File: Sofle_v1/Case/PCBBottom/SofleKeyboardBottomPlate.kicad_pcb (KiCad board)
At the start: 2 copper layers, 137.2 x 109.2 mm, 9 parts

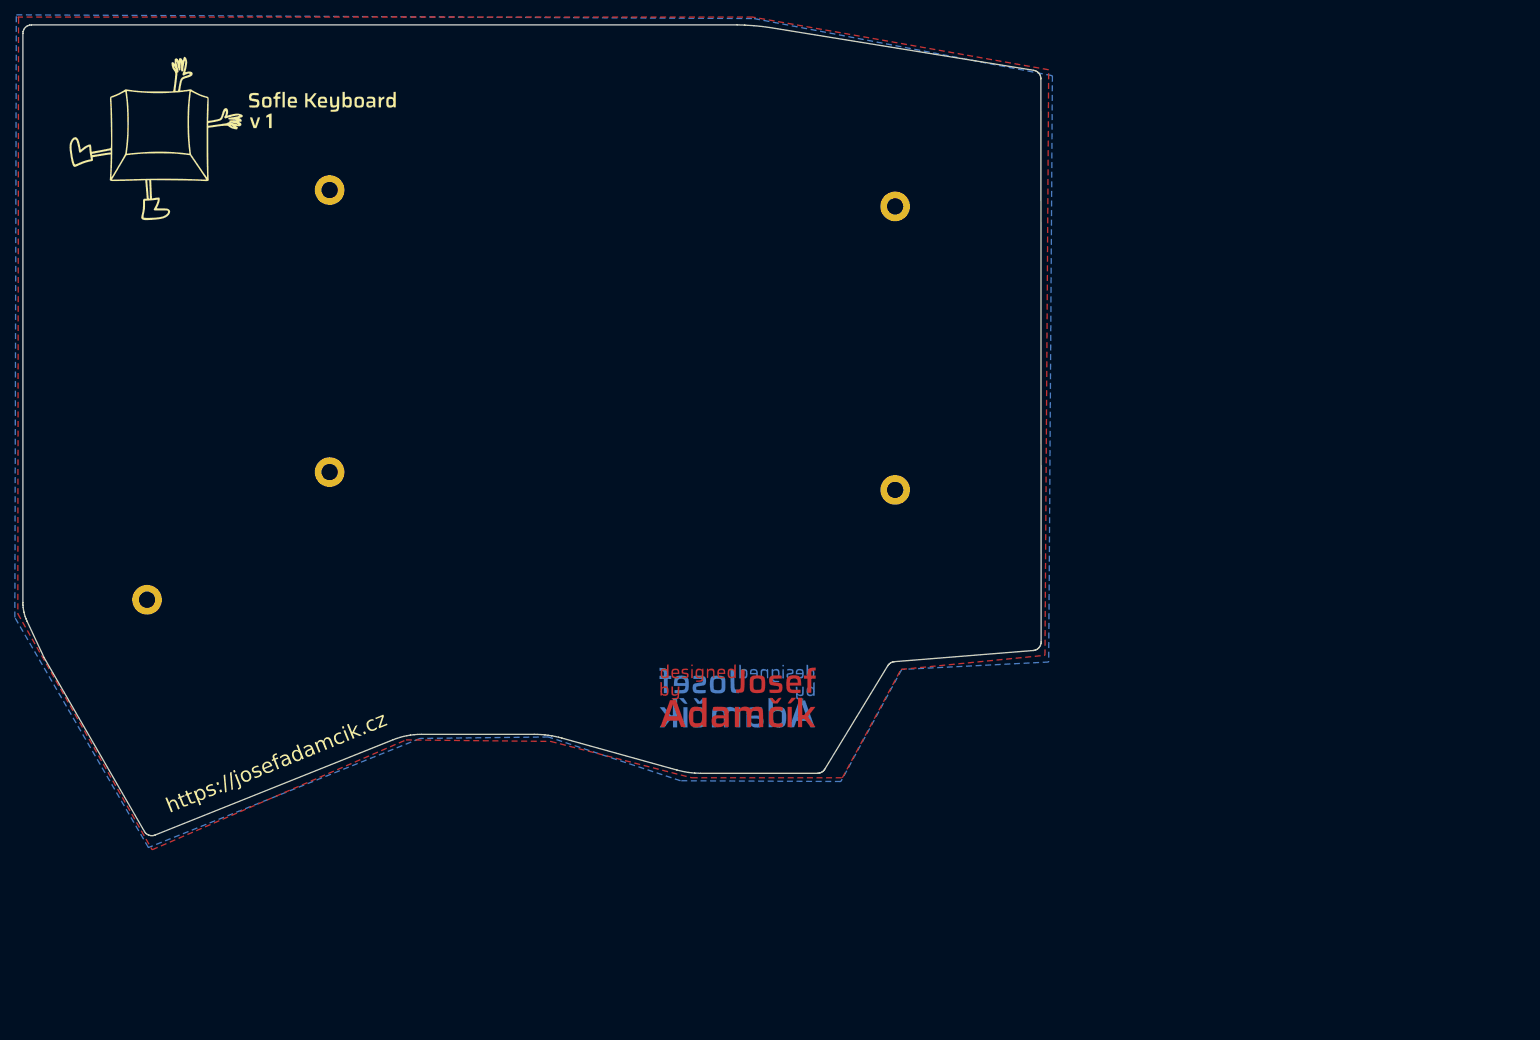
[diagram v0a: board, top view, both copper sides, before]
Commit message: Plates.
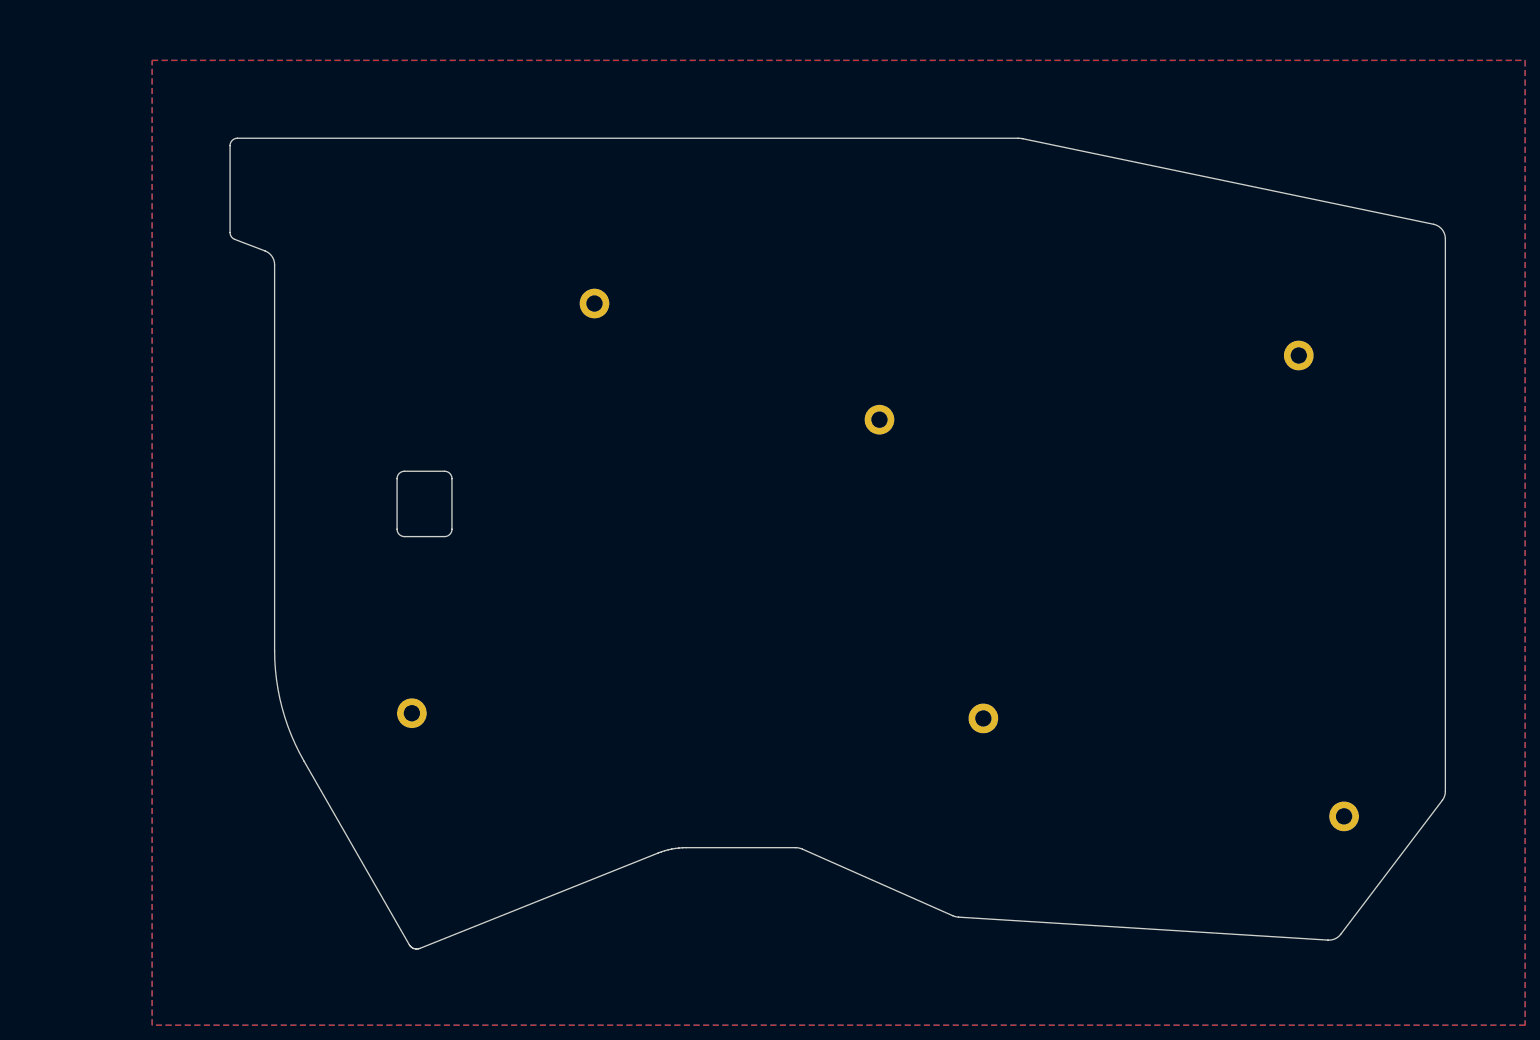
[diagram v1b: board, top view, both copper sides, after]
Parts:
- removed ? (x5): , Wire_Pads:SolderWirePad_single_0-8mmDrill
- removed the Ref** at (117.2, 114.0)
- removed the Ref** at (116.6, 113.9)
- removed the Ref** at (37.0, 38.6)
- removed the Ref** at (40.6, 39.0)
- added Ref**: Val**, SofleKeyboard:Sofle_Signature_DStasio, F.Cu at (174.0, 136.0)
- added Ref**: Val**, SofleKeyboard:Sofle_Signature_DStasio, B.Cu at (174.3, 136.0)
- added TH3: HOLE, SofleKeyboard:SolderWirePad_single_0-8mmDrill, F.Cu at (97.6, 57.1)
- added TH4: HOLE, SofleKeyboard:SolderWirePad_single_0-8mmDrill, F.Cu at (192.5, 64.1)
- added TH5: HOLE, SofleKeyboard:SolderWirePad_single_0-8mmDrill, F.Cu at (136.0, 72.8)
- added TH6: HOLE, SofleKeyboard:SolderWirePad_single_0-8mmDrill, F.Cu at (198.6, 126.2)
- added TH7: HOLE, SofleKeyboard:SolderWirePad_single_0-8mmDrill, F.Cu at (73.0, 112.3)
- added TH8: HOLE, SofleKeyboard:SolderWirePad_single_0-8mmDrill, F.Cu at (150.0, 113.0)
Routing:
- added copper zone on B.Cu, net GND
- added copper zone on F.Cu, net GND
- removed copper zone on B.Cu, net (none)
- removed copper zone on F.Cu, net (none)
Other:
- board size 137.2 x 109.2 mm -> 163.8 x 109.2 mm
- net class Default removed
- board text removed: "https://josefadamcik.cz"
